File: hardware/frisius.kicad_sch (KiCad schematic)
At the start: 0 parts

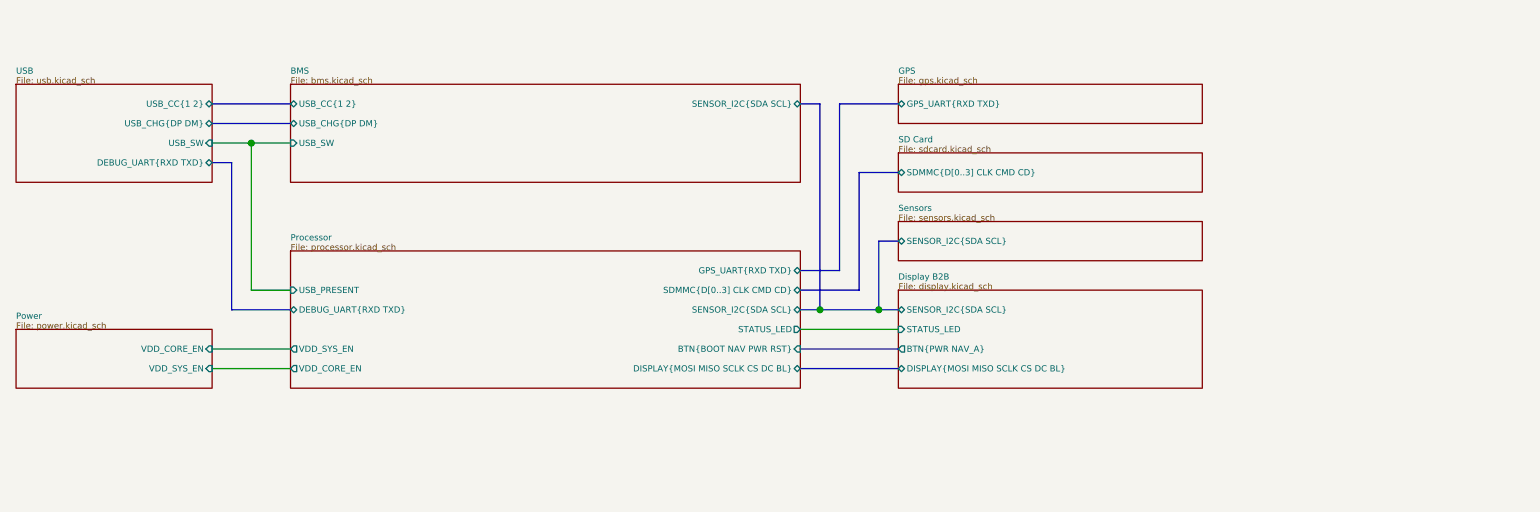
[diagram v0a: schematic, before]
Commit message: train schematics
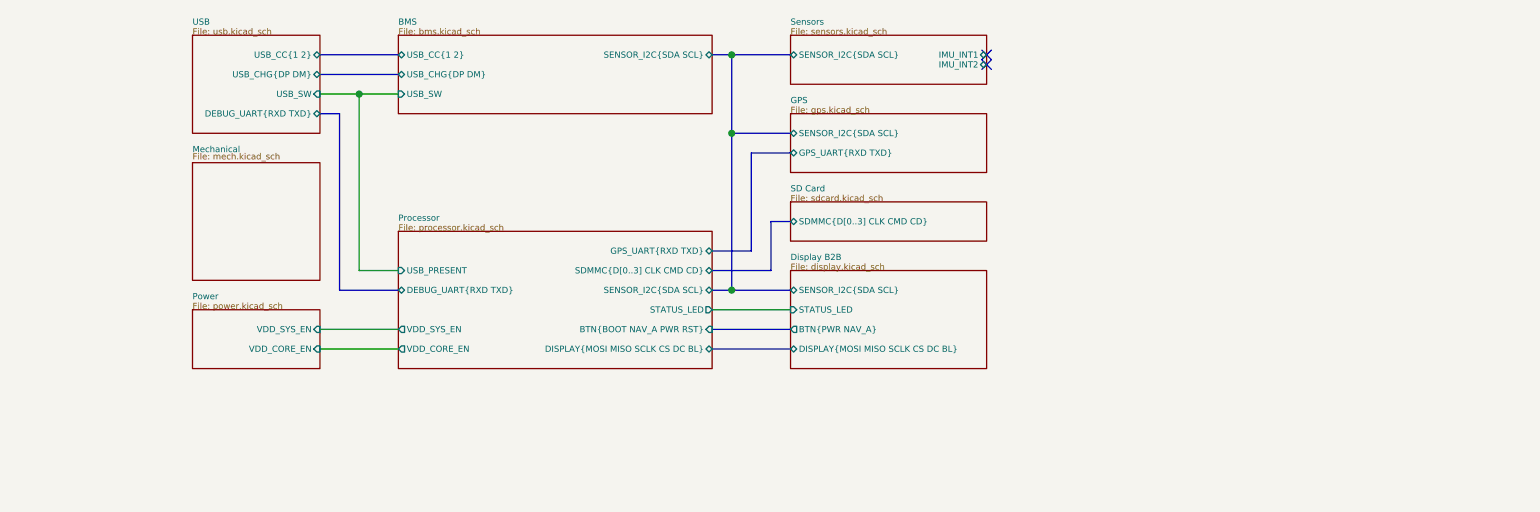
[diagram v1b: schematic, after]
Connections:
- no-connect marks 0 -> 2
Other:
- added sheet Mechanical (mech.kicad_sch)
- sheet GPS ports: added SENSOR_I2C{SDA SCL}; removed none
- sheet Processor ports: added BTN{BOOT NAV_A PWR RST}; removed BTN{BOOT NAV PWR RST}
- sheet Sensors ports: added IMU_INT1, IMU_INT2; removed none
- company: Erdapfel -> Frisius

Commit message: usb, charger, sensors, heir
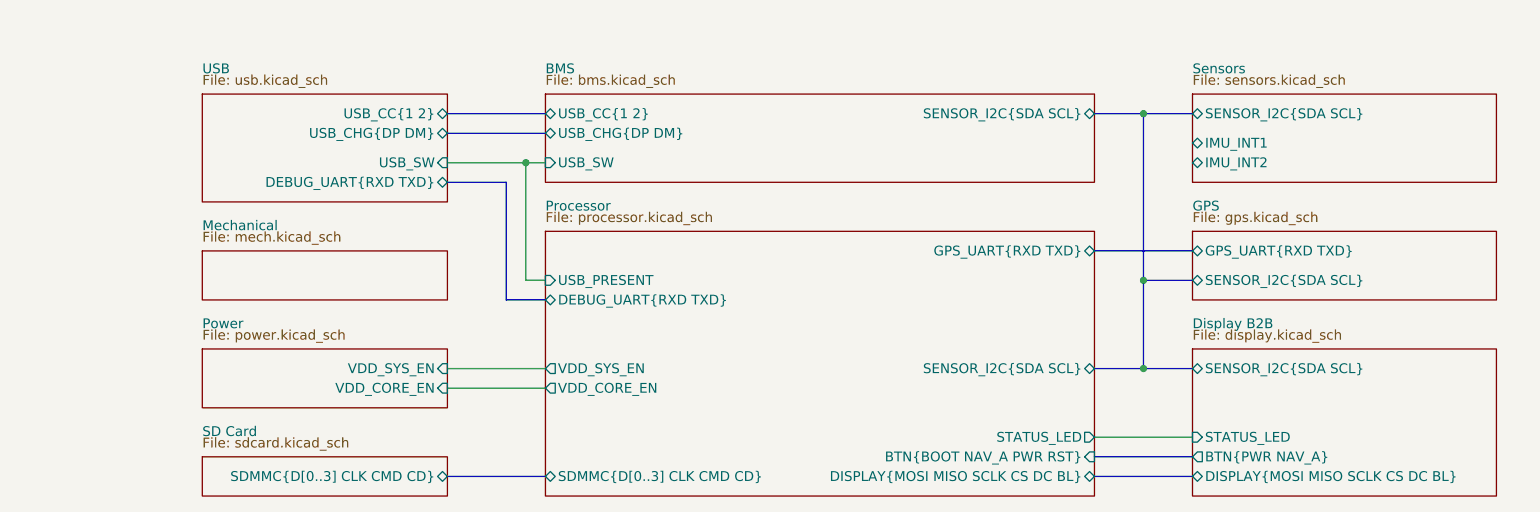
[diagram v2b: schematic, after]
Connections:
- no-connect marks 2 -> 0
